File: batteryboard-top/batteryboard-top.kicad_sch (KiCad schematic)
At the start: 6 parts, among them J1 Conn_02x05_Odd_Even, J2 Conn_02x05_Odd_Even

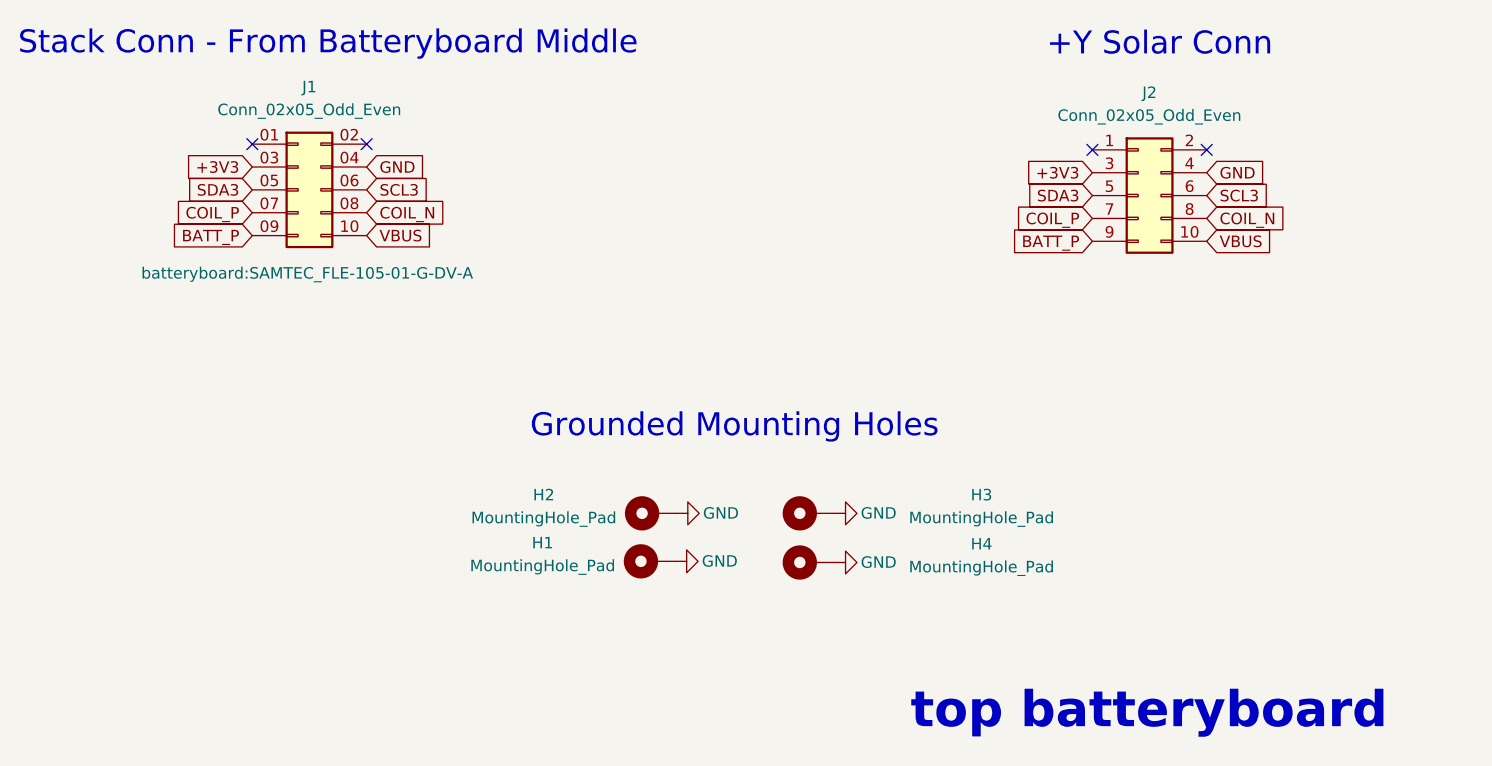
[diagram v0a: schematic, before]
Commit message: Recheck boards and re-export models
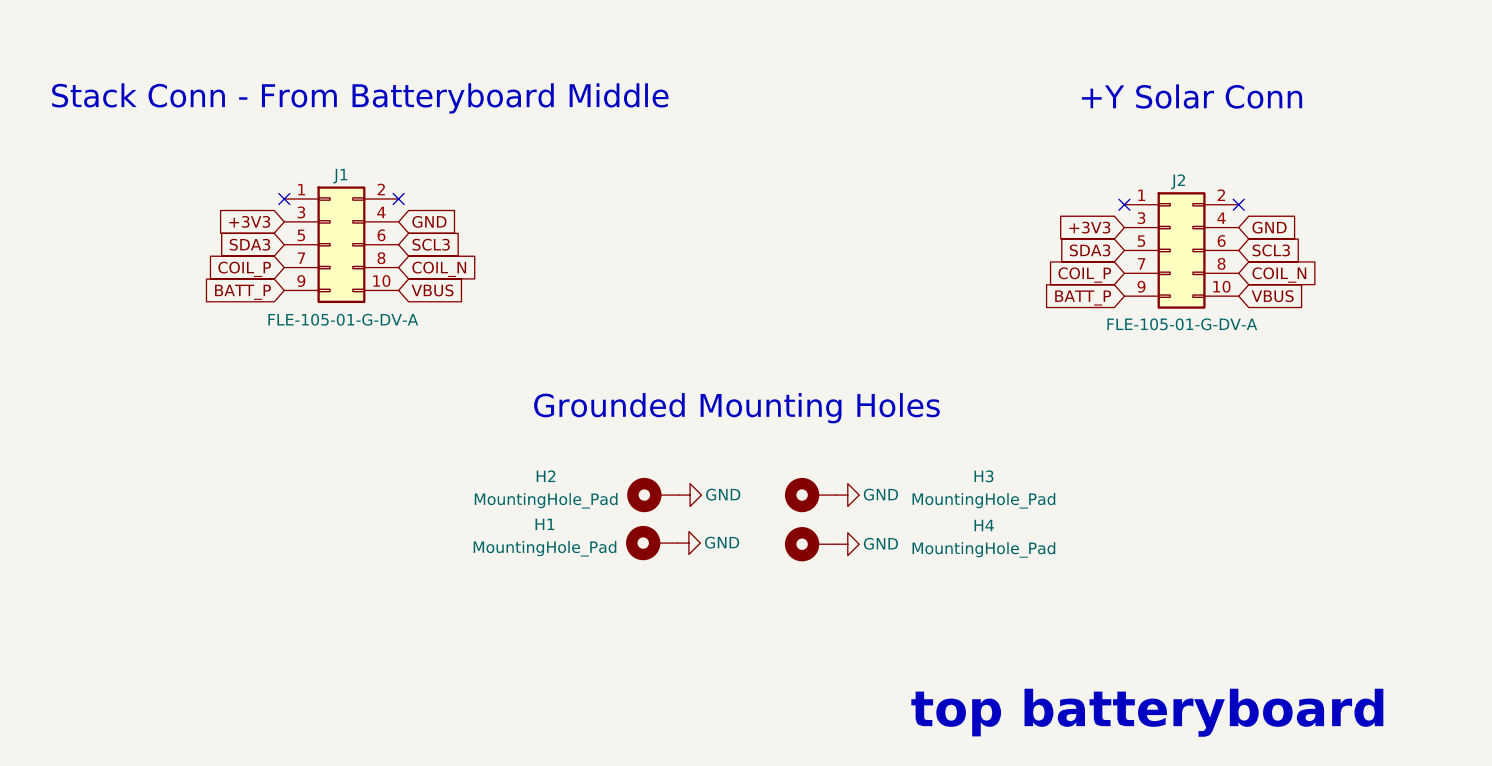
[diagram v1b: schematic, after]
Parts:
- J1: value Conn_02x05_Odd_Even -> FLE-105-01-G-DV-A
- J2: value Conn_02x05_Odd_Even -> FLE-105-01-G-DV-A; footprint batteryboard:FTS-105-XX-YY-DV-A -> batteryboard:SAMTEC_FLE-105-01-G-DV-A
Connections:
- net +3V3: now also J1.3 (Pin_3); no longer J1.03 (Pin_3)
- net BATT_P: now also J1.9 (Pin_9); no longer J1.09 (Pin_9)
- net COIL_N: now also J1.8 (Pin_8); no longer J1.08 (Pin_8)
- net COIL_P: now also J1.7 (Pin_7); no longer J1.07 (Pin_7)
- net GND: now also J1.4 (Pin_4); no longer J1.04 (Pin_4)
- net SCL3: now also J1.6 (Pin_6); no longer J1.06 (Pin_6)
- net SDA3: now also J1.5 (Pin_5); no longer J1.05 (Pin_5)
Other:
- moved on the sheet: H1, H2, H3, H4, J1, J2
